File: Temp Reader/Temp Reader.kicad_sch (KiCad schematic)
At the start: 3 parts, among them U1 ESP32-WROOM-32, U2 BME280, U4 NRF24L01_Breakout

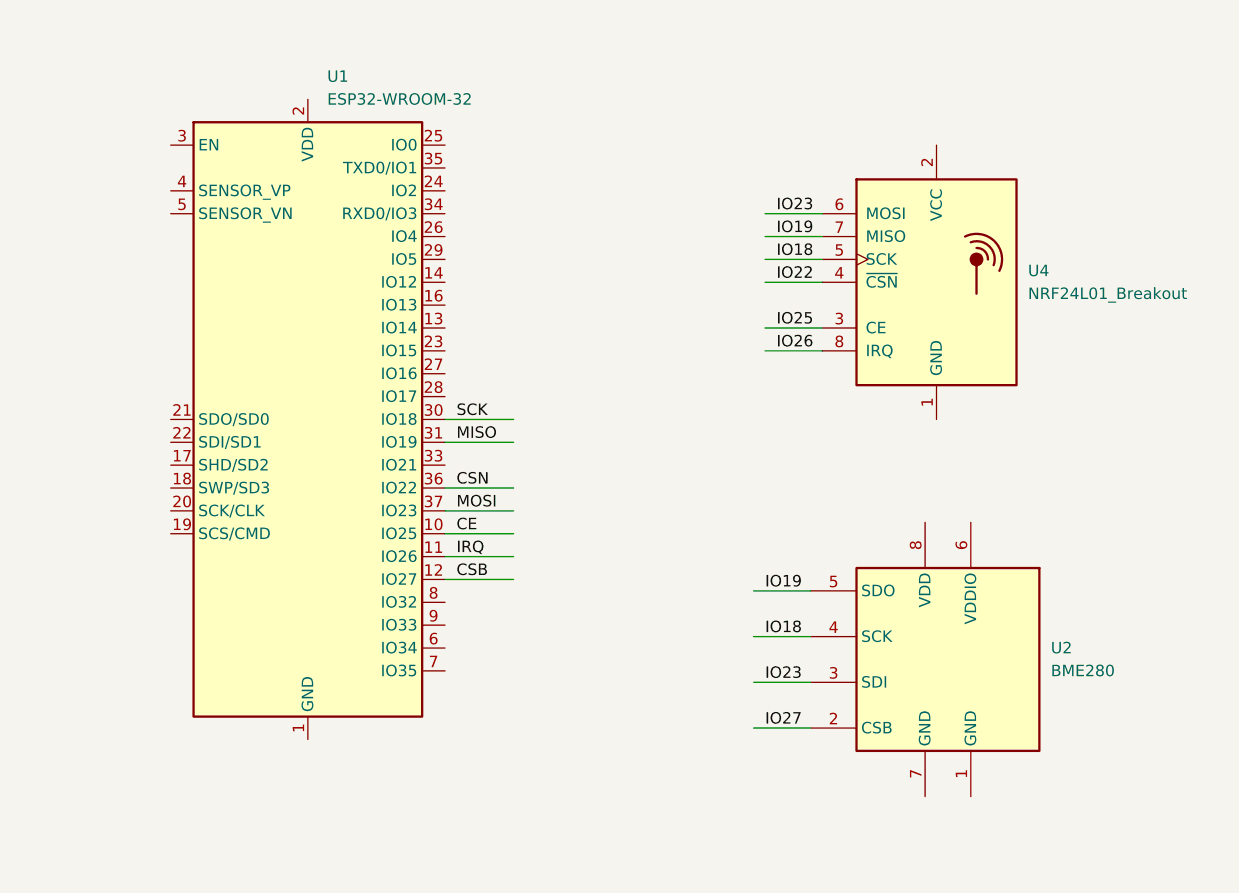
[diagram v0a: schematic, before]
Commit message: 2.First Schematic Look
No Buck

Raw schematic
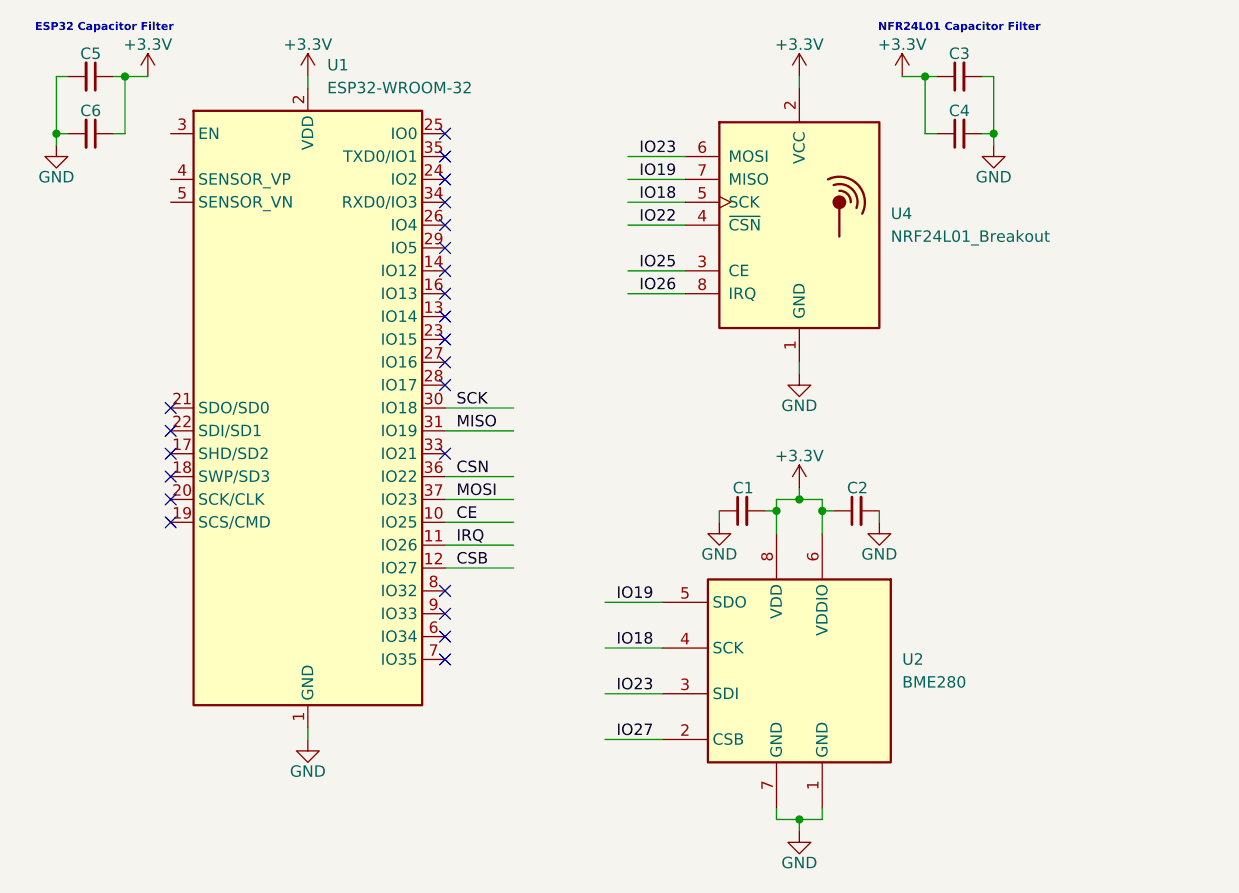
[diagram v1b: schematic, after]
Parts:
- added C1, C2, C3, C5: 100nF, symbol Device:C_Small
- added C4, C6: 10uF, symbol Device:C_Small
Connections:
- net GND: now reaches U4.1 (GND)
- net GND: now also U1.1 (GND), U1.15 (GND), U1.38 (GND), U1.39 (GND), U2.1 (GND), U2.7 (GND), C1.1, C2.2, C3.2, C4.2, C5.2, C6.2
- net +3.3V: now reaches U4.2 (VCC)
- net +3.3V: now also U1.2 (VDD), U2.6 (VDDIO), U2.8 (VDD), C1.2, C2.1, C3.1, C4.1, C5.1, C6.1
- no-connect marks 0 -> 23
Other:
- note added: "ESP32 Capacitor Filter"
- note added: "NFR24L01 Capacitor Filter"
- moved on the sheet: U1, U2, U4

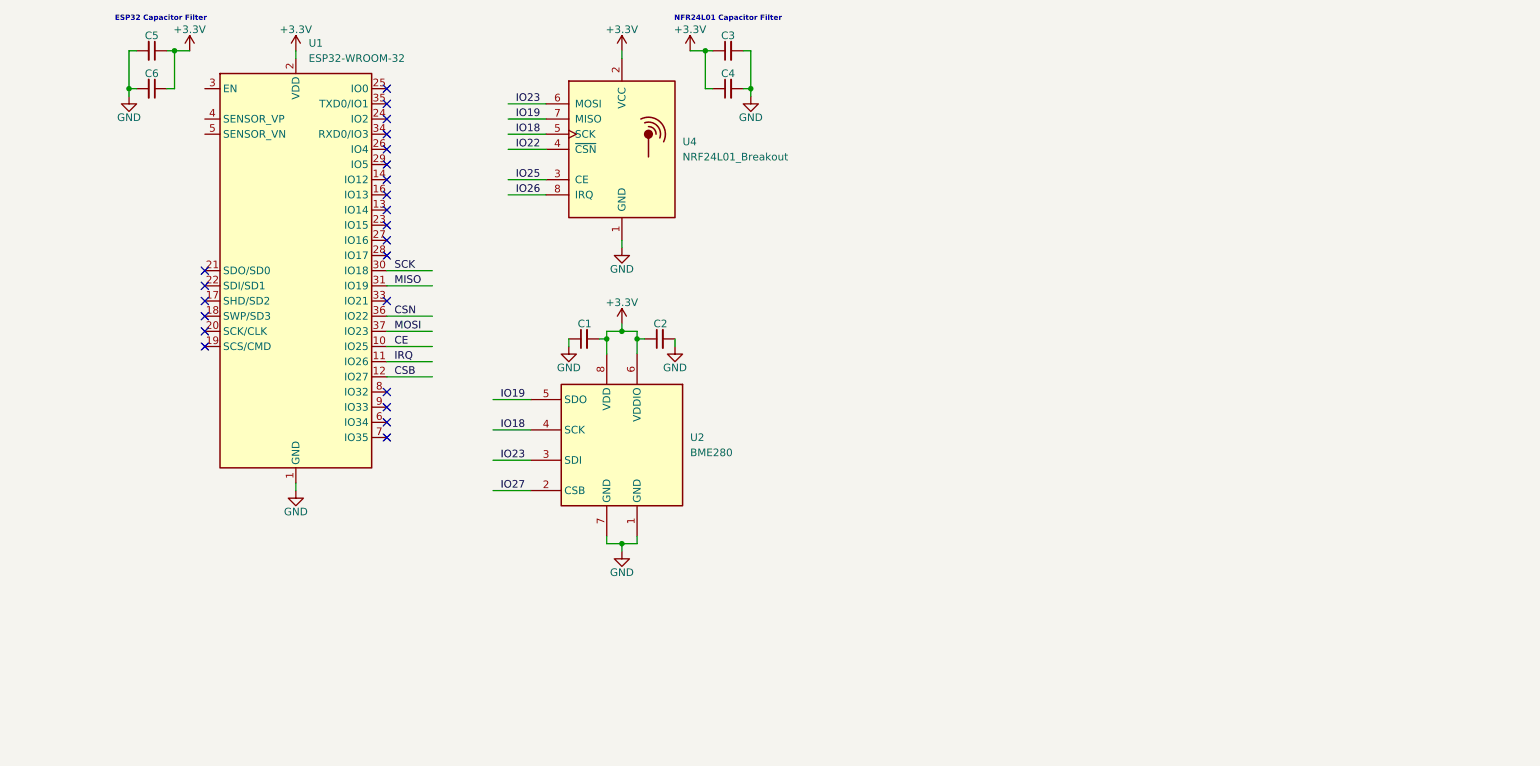
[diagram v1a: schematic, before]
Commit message: 3. 80% schematic done
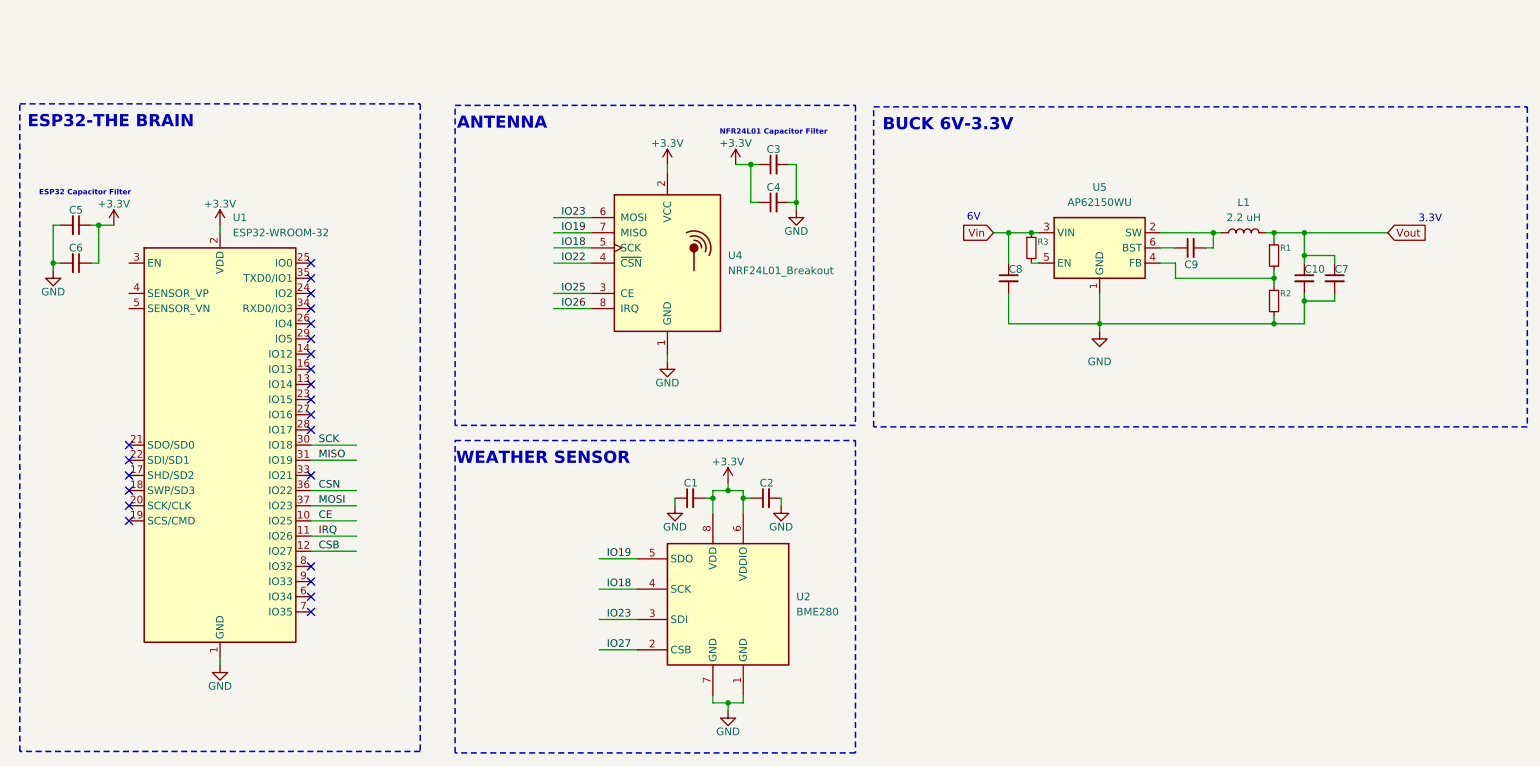
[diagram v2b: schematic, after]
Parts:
- added C10, C7, C8: 22uF, symbol Device:C_Small
- added C9: 100nF, symbol Device:C_Small
- added L1: 2.2 uH, symbol Device:L
- added R1: 31.25k, symbol Device:R_Small
- added R2: 10k, symbol Device:R_Small
- added R3: 100k, symbol Device:R_Small
- added U5: AP62150WU, Package_TO_SOT_SMD:TSOT-23-6, symbol Regulator_Switching:AP62150WU
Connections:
- net GND: now also C10.2, C7.2, C8.2, R2.2, U5.1 (GND)
- new net: C9.1, U5.6 (BST)
- new net: C9.2, L1.1, U5.2 (SW)
- new net: R1.2, R2.1, U5.4 (FB)
- new net: R3.2, U5.5 (EN)
- new net Vin: C8.1, R3.1, U5.3 (VIN)
- new net Vout: C10.1, C7.1, L1.2, R1.1
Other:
- note added: "3.3V"
- note added: "6V"
- note added: "ANTENNA"
- note added: "BUCK 6V-3.3V"
- note added: "ESP32-THE BRAIN"
- note added: "WEATHER SENSOR"
- moved on the sheet: C1, C2, C3, C4, C5, C6, U1, U2, U4
